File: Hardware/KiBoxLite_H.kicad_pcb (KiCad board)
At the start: 4 copper layers, 49.6 x 86.5 mm, 161 parts, among them J1 Screw_Terminal_01x03, J2 USB4105-GF-A-060, J3 RJ45_Abracon_ARJP11A-MASA-B-A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, Q2 BC817-40(SOT23), Q3 BC817-40(SOT23), T1 LMUN2211LT1G(SOT-23), U1 CH340X(MSOP-10), U10 MAX13487, U3 TP4054-42-SOT25-R(SOT23-5), U4 LAN8710A-EZC(QFN32), U5 TX4138(ESOIC-8), U6 ESP32-WROOM-32E-N4, U7 TPS62A02ADRLR(SOT-563-6), U8 NA(SN74LVC1G04DBVR(SOT23-5)), U9 TPS2378DDAR(HSOIC-8)

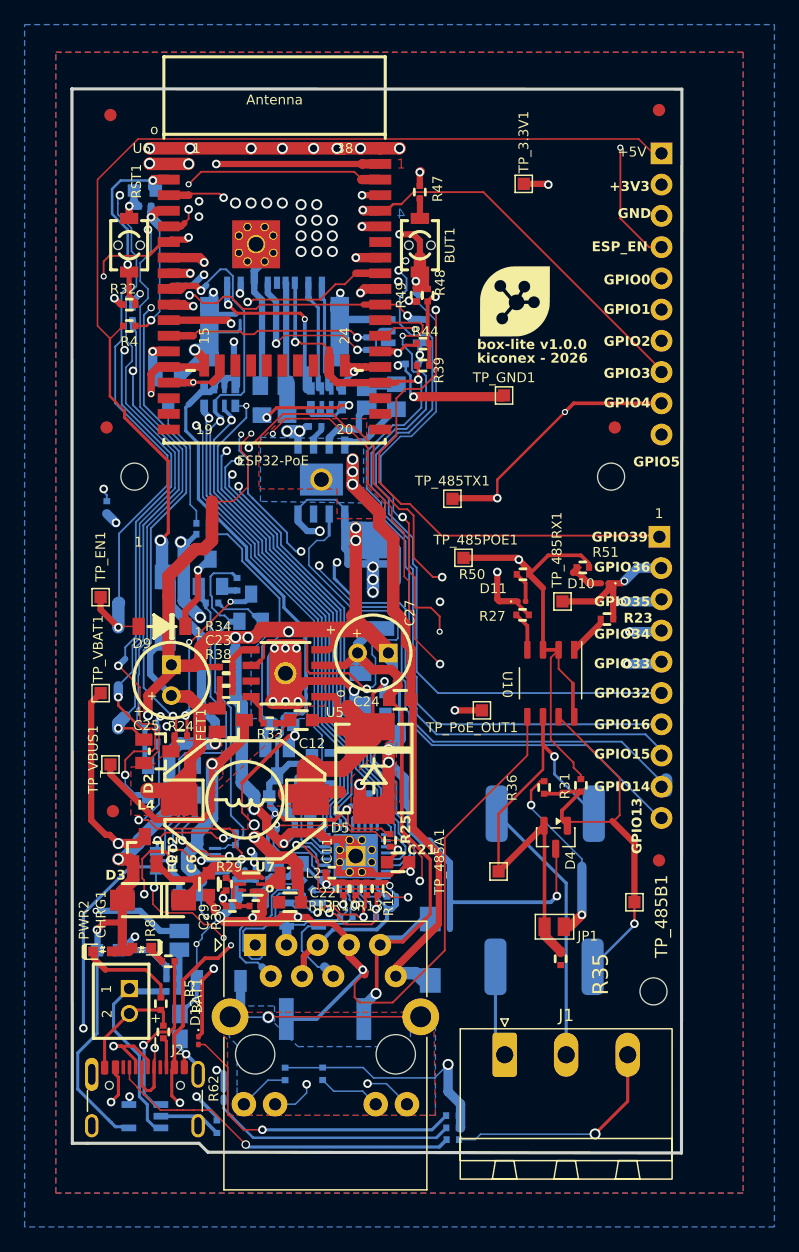
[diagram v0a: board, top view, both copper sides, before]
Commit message: build: optimizacion pcb
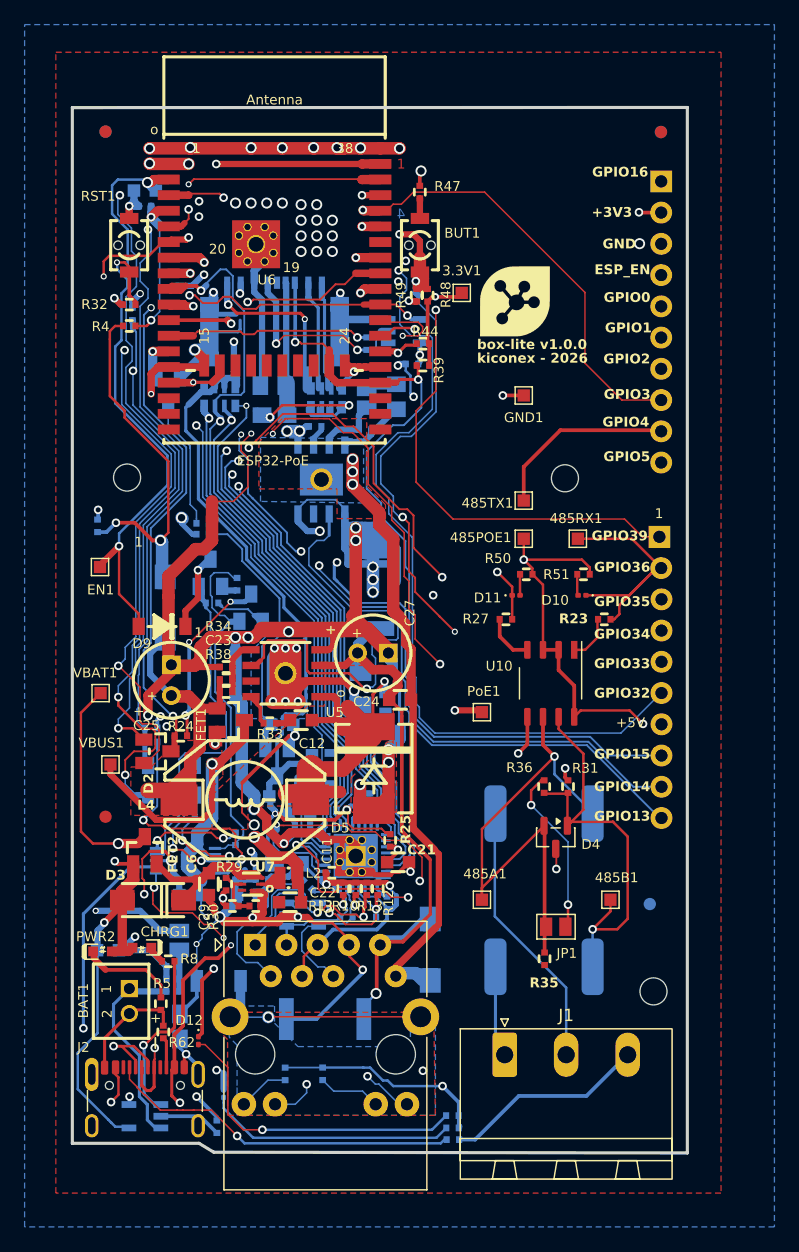
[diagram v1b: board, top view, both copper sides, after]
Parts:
- FID2, FID5, FID6: moved to B.Cu
- moved FID5 24.3 mm to (135.6, 90.0), turned to 180 degrees
- moved FID2 24.0 mm to (90.4, 90.0), turned to 180 degrees
- moved 3.3V1 10.2 mm to (119.4, 103.1)
- moved 485TX1 5.80 mm to (124.4, 120.0)
- moved 485RX1 5.25 mm to (128.8, 123.0)
- moved 485POE1 5.14 mm to (124.4, 123.0)
- moved MH2 3.75 mm to (127.8, 118.1)
- moved FID6 3.63 mm to (134.7, 152.8), turned to 180 degrees
- moved 485A1 2.67 mm to (121.0, 152.4)
- moved EN1 2.45 mm to (90.0, 125.3)
- moved EXT1 2.28 mm to (135.6, 105.4)
- moved D10 2.09 mm to (129.1, 127.7)
- moved 485B1 1.96 mm to (131.4, 152.4)
- moved FID3 1.79 mm to (135.6, 90.0)
- moved R1 1.67 mm to (89.8, 122.0)
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- renumbered TP_3.3V1 to 3.3V1, TP_485A1 to 485A1, TP_485B1 to 485B1, TP_485POE1 to 485POE1, TP_485RX1 to 485RX1, TP_485TX1 to 485TX1, TP_EN1 to EN1, TP_GND1 to GND1, TP_PoE_OUT1 to PoE1, TP_VBAT1 to VBAT1, TP_VBUS1 to VBUS1
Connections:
- EXT1 pad 1: +5V -> /GPIO16\I2C-SCL
- EXT2 pad 7: /GPIO16\I2C-SCL -> +5V
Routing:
- net +5V: track 227.7 -> 96.0 mm, vias 6 -> 8
- net GND: track 526.3 -> 448.3 mm, vias 63 -> 66
- net +3.3V: track 277.4 -> 205.0 mm, vias 15 -> 14
- net /GPIO16\I2C-SCL: track 85.4 -> 55.5 mm
- net /485_TX: track 53.6 -> 68.6 mm, vias 4 -> 2
- net /GPIO5\SPI_CS: track 67.6 -> 54.2 mm
- net /485_RX: track 84.1 -> 95.6 mm, vias 4 -> 3
- net /GPI39: track 78.7 -> 73.7 mm
- net /GPIO3\U0RXD: track 103.2 -> 108.0 mm
- net /GPIO32: track 79.8 -> 84.2 mm
- net /TD+: track 25.0 -> 21.8 mm
- net /ESP_EN: track 106.1 -> 109.1 mm, vias 4 -> 3
- net /GPIO0: track 97.0 -> 95.0 mm
- net Net-(D10-A): track 3.51 -> 1.74 mm
- net /GPI34\BUT1: track 85.9 -> 84.1 mm, vias 6 -> 5
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- added copper zone on In2.Cu, net +5V
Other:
- board size 49.6 x 86.5 mm -> 50 x 85 mm
